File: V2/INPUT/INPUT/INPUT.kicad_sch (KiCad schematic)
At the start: 54 parts, among them J1 Conn_01x03, J2 USB_C_Receptacle_USB2.0_16P, J3 Conn_01x03, J4 Conn_01x03, J5 Conn_01x03, J6 Conn_01x03, J7 Conn_01x03, J8 Conn_01x03, J9 Conn_01x03, Q1 QM6006D, Q2 QM6006D, Q3 QM6006D, Q4 QM6006D, Q5 QM6006D, Q6 QM6006D, Q7 QM6006D, Q8 QM6006D, SW1 SW_SPST, SW2 SW_SPST, SW3 SW_SPST, SW4 SW_SPST, SW5 SW_SPST, SW6 SW_SPST, SW7 SW_SPST, SW8 SW_SPST, U1 USBLC6-2P6

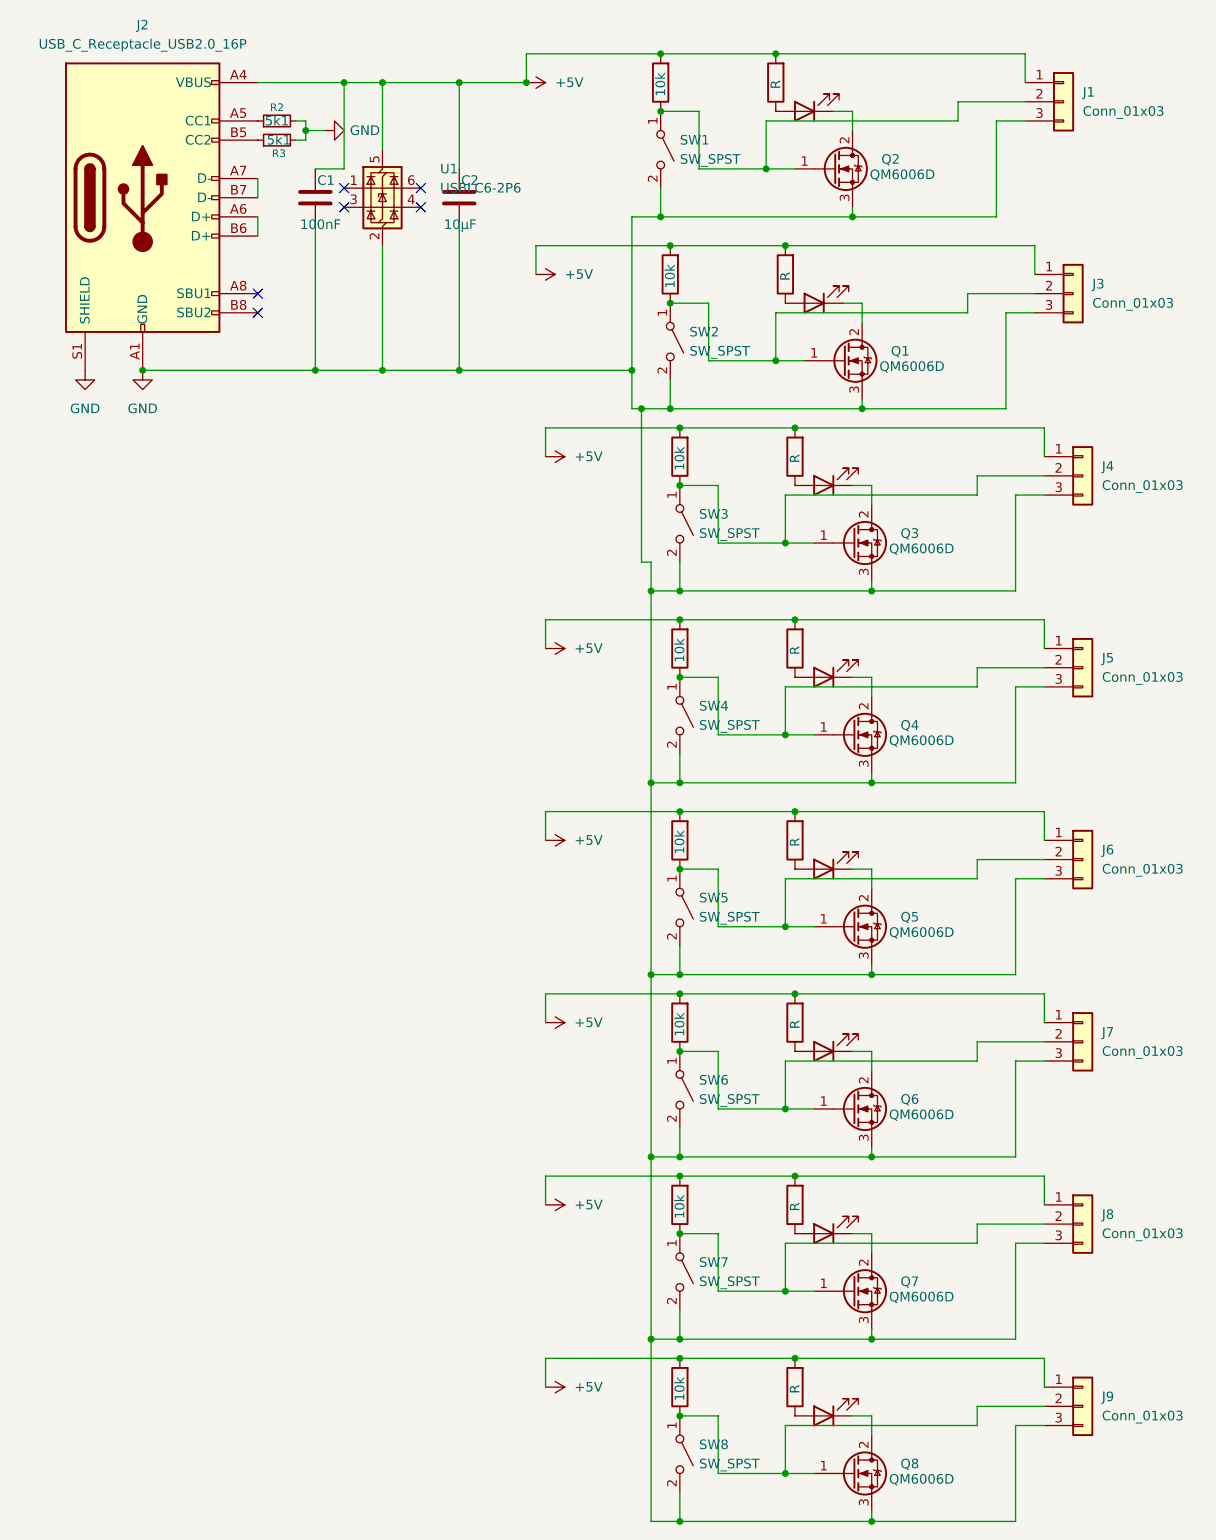
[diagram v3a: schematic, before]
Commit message: Auto-update: 28.03.2026  0:16:29,83
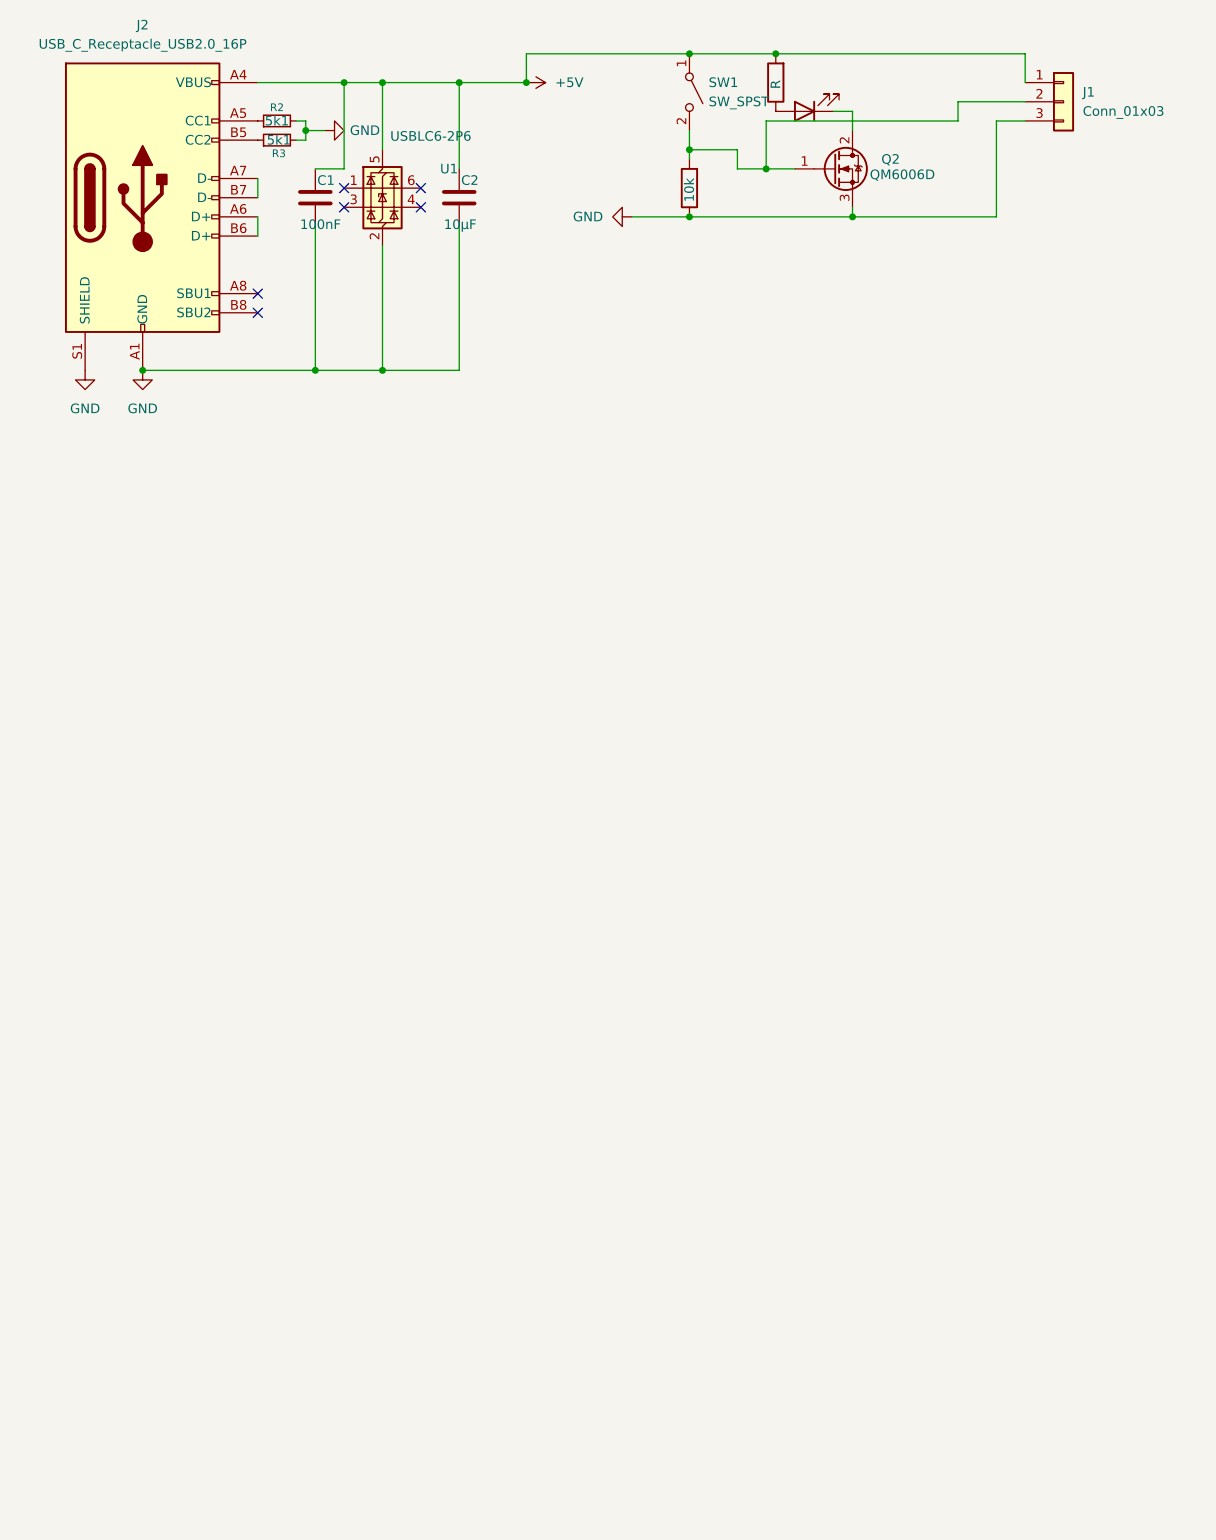
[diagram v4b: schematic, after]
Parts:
- removed D2, D3, D4, D5, D6, D7, D8: LED, LED_SMD:LED_1206_3216Metric, symbol Device:LED
- removed J3, J4, J5, J6, J7, J8, J9: Conn_01x03, Connector_PinSocket_2.54mm:PinSocket_1x03_P2.54mm_Horizontal, symbol Connector_Generic:Conn_01x03
- removed Q1, Q3, Q4, Q5, Q6, Q7, Q8: QM6006D, Package_TO_SOT_SMD:SOT-23, symbol Transistor_FET:QM6006D
- removed R10, R12, R14, R16, R18, R6, R8: R, Resistor_SMD:R_0201_0603Metric, symbol Device:R
- removed R11, R13, R15, R17, R5, R7, R9: 10k, Resistor_SMD:R_0201_0603Metric, symbol Device:R
- removed SW2, SW3, SW4, SW5, SW6, SW7, SW8: SW_SPST, Button_Switch_THT:SW_Slide-03_Wuerth-WS-SLTV_10x2.5x6.4_P2.54mm, symbol Switch:SW_SPST
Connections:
- net +5V: now also SW1.1 (A); no longer R4.2
- net GND: now also R4.1; no longer SW1.2 (B)
- net at J1.2 (Pin_2), Q2.1 (G): now also R4.2, SW1.2 (B); no longer R4.1, SW1.1 (A)
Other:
- moved on the sheet: SW1
